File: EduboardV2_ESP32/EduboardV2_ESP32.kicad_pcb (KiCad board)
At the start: 2 copper layers, 30 x 51 mm, 19 parts, among them J1 Conn_02x26_Odd_Even, Q1 S8050_C139514, Q2 S8050_C139514, SW1 K2-1102SP-C4SC-04, SW2 K2-1102SP-C4SC-04, U1 ESP32-WROOM-E, U2 FT2232HL, U3 M93C46-WMN6TP

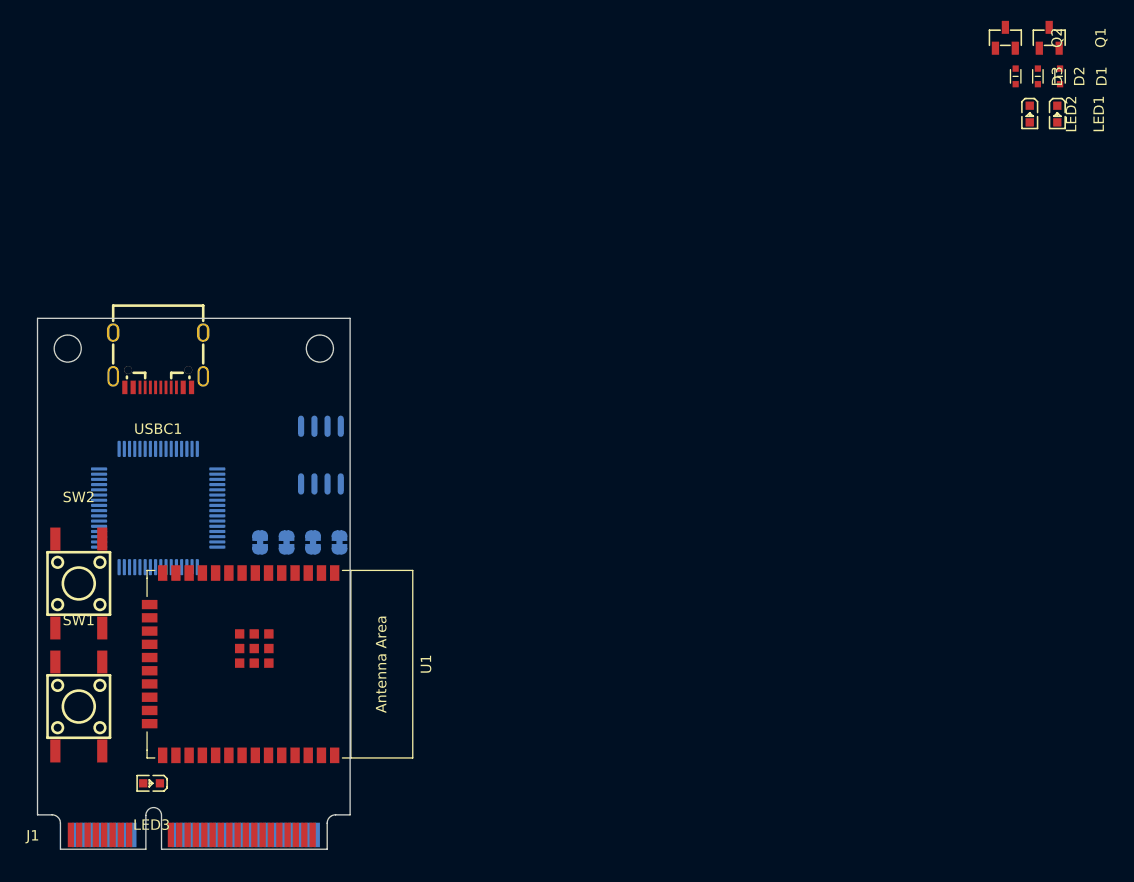
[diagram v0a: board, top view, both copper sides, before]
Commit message: all parts placed. descision about usb-debug line to be made...
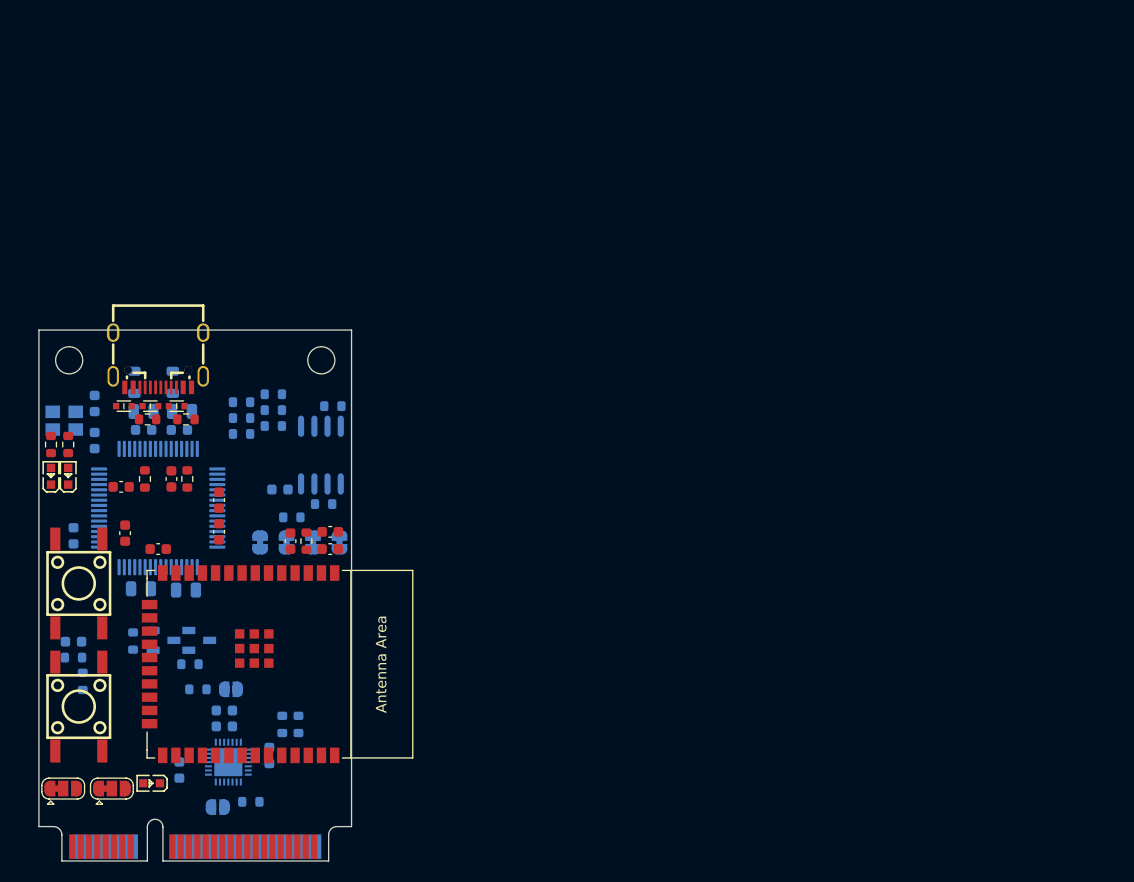
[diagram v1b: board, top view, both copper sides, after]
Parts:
- added C1: 12p, Capacitor_SMD:C_0603_1608Metric, B.Cu at (109.7, 113.5)
- added C10: 100n, Capacitor_SMD:C_0603_1608Metric, F.Cu at (117.1, 120.8)
- added C11: 100n, Capacitor_SMD:C_0603_1608Metric, F.Cu at (112.3, 121.5)
- added C12: 100n, Capacitor_SMD:C_0603_1608Metric, B.Cu at (107.7, 126.2)
- added C13: 100n, Capacitor_SMD:C_0603_1608Metric, F.Cu at (112.6, 126.0)
- added C14: 100n, Capacitor_SMD:C_0603_1608Metric, F.Cu at (121.7, 122.8)
- added C15: 100n, Capacitor_SMD:C_0603_1608Metric, F.Cu at (121.7, 125.9)
- added C16: 100n, Capacitor_SMD:C_0603_1608Metric, F.Cu at (115.8, 127.5)
- added C17: 100n, Capacitor_SMD:C_0603_1608Metric, F.Cu at (128.5, 126.7)
- added C18: 100n, Capacitor_SMD:C_0603_1608Metric, B.Cu at (107.7, 136.4)
- added C19: 100n, Capacitor_SMD:C_0603_1608Metric, F.Cu at (132.3, 127.5)
- added C2: 12p, Capacitor_SMD:C_0603_1608Metric, B.Cu at (109.7, 117.1)
- added C20: 1u, Capacitor_SMD:C_0603_1608Metric, F.Cu at (132.3, 125.9)
- added C21: 1u, Capacitor_SMD:C_0603_1608Metric, B.Cu at (122.2, 143.0)
- added C22: 100n, Capacitor_SMD:C_0603_1608Metric, B.Cu at (122.2, 144.5)
- added C23: 100n, Capacitor_SMD:C_0603_1608Metric, B.Cu at (117.9, 148.7)
- added C24: 100n, Capacitor_SMD:C_0603_1608Metric, B.Cu at (126.5, 147.3)
- added C3: 100n, Capacitor_SMD:C_0603_1608Metric, B.Cu at (127.5, 121.8)
- added C4: 4u7, Capacitor_SMD:C_0805_2012Metric, B.Cu at (118.5, 131.4)
- added C5: 4u7, Capacitor_SMD:C_0805_2012Metric, B.Cu at (114.2, 131.3)
- added C6: 4u7, Capacitor_SMD:C_0805_2012Metric, B.Cu at (114.4, 114.3)
- added C7: 4u7, Capacitor_SMD:C_0805_2012Metric, B.Cu at (118.1, 114.3)
- added C8: 100n, Capacitor_SMD:C_0603_1608Metric, B.Cu at (117.9, 116.1)
- added C9: 100n, Capacitor_SMD:C_0603_1608Metric, B.Cu at (114.4, 116.1)
- added FB1: FerriteBead_Small, Inductor_SMD:L_0805_2012Metric, B.Cu at (117.2, 111.5)
- added FB2: FerriteBead_Small, Inductor_SMD:L_0805_2012Metric, B.Cu at (113.5, 111.5)
- added JP5: SolderJumper_2_Open, Jumper:SolderJumper-2_P1.3mm_Open_RoundedPad1.0x1.5mm, B.Cu at (121.5, 152.3)
- added JP6: SolderJumper_2_Open, Jumper:SolderJumper-2_P1.3mm_Open_RoundedPad1.0x1.5mm, B.Cu at (122.8, 141.0)
- added JP7: SolderJumper_3_Bridged12, Jumper:SolderJumper-3_P1.3mm_Bridged12_RoundedPad1.0x1.5mm, F.Cu at (111.4, 150.5)
- added JP8: SolderJumper_3_Bridged12, Jumper:SolderJumper-3_P1.3mm_Bridged12_RoundedPad1.0x1.5mm, F.Cu at (106.7, 150.5)
- added R1: 2k2, Resistor_SMD:R_0603_1608Metric, B.Cu at (132.6, 113.8)
- added R10: 33R, Resistor_SMD:R_0603_1608Metric, B.Cu at (123.8, 116.5)
- added R11: 33R, Resistor_SMD:R_0603_1608Metric, B.Cu at (123.8, 114.9)
- added R12: 33R, Resistor_SMD:R_0603_1608Metric, B.Cu at (123.8, 113.4)
- added R13: 2k2, Resistor_SMD:R_0603_1608Metric, F.Cu at (107.2, 117.5)
- added R14: 2k2, Resistor_SMD:R_0603_1608Metric, F.Cu at (105.5, 117.5)
- added R15: 0R, Resistor_SMD:R_0603_1608Metric, B.Cu at (129.3, 144.3)
- added R16: 0R, Resistor_SMD:R_0603_1608Metric, B.Cu at (127.7, 144.3)
- added R17: 10k, Resistor_SMD:R_0603_1608Metric, B.Cu at (113.4, 136.3)
- added R18: 10k, Resistor_SMD:R_0603_1608Metric, B.Cu at (118.9, 138.6)
- added R19: 10k, Resistor_SMD:R_0603_1608Metric, F.Cu at (130.0, 126.7)
- added R2: 10k, Resistor_SMD:R_0603_1608Metric, B.Cu at (126.9, 114.2)
- added R20: 10k, Resistor_SMD:R_0603_1608Metric, B.Cu at (107.7, 137.9)
- added R21: 0R, Resistor_SMD:R_0603_1608Metric, B.Cu at (131.7, 123.2)
- added R22: 2k2, Resistor_SMD:R_0603_1608Metric, B.Cu at (108.6, 140.2)
- added R23: 10k, Resistor_SMD:R_0603_1608Metric, B.Cu at (124.7, 151.8)
- added R24: 10k, Resistor_SMD:R_0603_1608Metric, B.Cu at (119.6, 141.0)
- added R3: 10k, Resistor_SMD:R_0603_1608Metric, B.Cu at (126.9, 112.6)
- added R4: 10k, Resistor_SMD:R_0603_1608Metric, B.Cu at (126.9, 115.7)
- added R5: 0R, Resistor_SMD:R_0603_1608Metric, B.Cu at (128.7, 124.5)
- added R6: 10k, Resistor_SMD:R_0603_1608Metric, F.Cu at (114.8, 115.1)
- added R7: 10k, Resistor_SMD:R_0603_1608Metric, F.Cu at (118.5, 115.1)
- added R8: 1k, Resistor_SMD:R_0603_1608Metric, F.Cu at (118.6, 120.8)
- added R9: 12k, Resistor_SMD:R_0603_1608Metric, F.Cu at (114.6, 120.8)
- added U4: SX1509BIULTRT, EduboardV2_kicadlib:QFN-28_L4.0-W4.0-P0.40-BL-EP, B.Cu at (122.6, 148.0)
- added Y2: 12MHz, Crystal:Crystal_SMD_3225-4Pin_3.2x2.5mm, B.Cu at (106.8, 115.2)
- J1: value Conn_02x26_Odd_Even -> EduboardV2 PCIE UP Board Connector; footprint mpcie:mini-PCIe_F1_Full -> EduboardV2_kicadlib:mini-PCIe_F1_Full
- Q1, Q2: moved to B.Cu
- moved LED1 101.1 mm to (107.2, 120.5), turned to 90 degrees
- moved LED2 100.2 mm to (105.5, 120.5), turned to 90 degrees
- moved Q1 100.0 mm to (119.8, 136.3), turned to 180 degrees
- moved Q2 99.4 mm to (116.3, 136.3), turned to 180 degrees
- moved D1 95.3 mm to (112.5, 113.8), turned to 0 degrees
- moved D3 88.9 mm to (115.1, 113.8), turned to 0 degrees
- moved D2 88.5 mm to (117.6, 113.8), turned to 180 degrees
- moved J1 1.14 mm to (115.5, 157.4)
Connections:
- J1 pad 1: unconnected-(J1-Pin_1-Pad1) -> GND
- J1 pad 10: unconnected-(J1-Pin_10-Pad10) -> USB_Debug_D-
- J1 pad 11: unconnected-(J1-Pin_11-Pad11) -> Net-(J1-UART0_UP_RX)
- J1 pad 12: unconnected-(J1-Pin_12-Pad12) -> USB_Debug_D+
- J1 pad 13: unconnected-(J1-Pin_13-Pad13) -> Net-(J1-UART1_RS485_TX)
- J1 pad 14: unconnected-(J1-Pin_14-Pad14) -> GND
- J1 pad 15: unconnected-(J1-Pin_15-Pad15) -> Net-(J1-UART1_RS485_RX)
- J1 pad 16: unconnected-(J1-Pin_16-Pad16) -> GPIO_RS485_DE
- J1 pad 17: unconnected-(J1-Pin_17-Pad17) -> ESP_TMS
- J1 pad 18: unconnected-(J1-Pin_18-Pad18) -> ESP_IO4
- J1 pad 19: unconnected-(J1-Pin_19-Pad19) -> ESP_TDI
- J1 pad 2: unconnected-(J1-Pin_2-Pad2) -> VBUS
- J1 pad 20: unconnected-(J1-Pin_20-Pad20) -> ESP_IO5
- J1 pad 21: unconnected-(J1-Pin_21-Pad21) -> ESP_TCK
- J1 pad 22: unconnected-(J1-Pin_22-Pad22) -> ESP_IO2
- J1 pad 23: unconnected-(J1-Pin_23-Pad23) -> ESP_TDO
- J1 pad 24: unconnected-(J1-Pin_24-Pad24) -> ESP_IO18
- J1 pad 25: unconnected-(J1-Pin_25-Pad25) -> GPIO_RotEnc_SW
- J1 pad 26: unconnected-(J1-Pin_26-Pad26) -> ESP_IO19
- J1 pad 27: unconnected-(J1-Pin_27-Pad27) -> ESP_IO33
- J1 pad 28: unconnected-(J1-Pin_28-Pad28) -> ESP_IO23
- J1 pad 29: unconnected-(J1-Pin_29-Pad29) -> ESP_IO27
- J1 pad 3: unconnected-(J1-Pin_3-Pad3) -> +5V
- J1 pad 30: unconnected-(J1-Pin_30-Pad30) -> ESP_IO22
- J1 pad 31: unconnected-(J1-Pin_31-Pad31) -> GPIO_PWM_R
- J1 pad 32: unconnected-(J1-Pin_32-Pad32) -> ESP_IO21
- J1 pad 33: unconnected-(J1-Pin_33-Pad33) -> GPIO_PWM_G
- J1 pad 34: unconnected-(J1-Pin_34-Pad34) -> ESP_IO0
- J1 pad 35: unconnected-(J1-Pin_35-Pad35) -> GPIO_PWM_B
- J1 pad 36: unconnected-(J1-Pin_36-Pad36) -> ESP_IO32
- J1 pad 37: unconnected-(J1-Pin_37-Pad37) -> GPIO_LED0
- J1 pad 38: unconnected-(J1-Pin_38-Pad38) -> ESP_IO25
- J1 pad 39: unconnected-(J1-Pin_39-Pad39) -> GPIO_LED1
- J1 pad 4: unconnected-(J1-Pin_4-Pad4) -> +5V
- J1 pad 40: unconnected-(J1-Pin_40-Pad40) -> ESP_IO35
- J1 pad 41: unconnected-(J1-Pin_41-Pad41) -> GPIO_LED2
- J1 pad 42: unconnected-(J1-Pin_42-Pad42) -> ESP_IO26
- J1 pad 43: unconnected-(J1-Pin_43-Pad43) -> GPIO_LED3
- J1 pad 44: unconnected-(J1-Pin_44-Pad44) -> ESP_IO36
- J1 pad 45: unconnected-(J1-Pin_45-Pad45) -> GPIO_LED4
- J1 pad 46: unconnected-(J1-Pin_46-Pad46) -> ESP_IO34
- J1 pad 47: unconnected-(J1-Pin_47-Pad47) -> GPIO_LED5
- J1 pad 48: unconnected-(J1-Pin_48-Pad48) -> ESP_IO39
- J1 pad 49: unconnected-(J1-Pin_49-Pad49) -> GPIO_LED6
- J1 pad 5: unconnected-(J1-Pin_5-Pad5) -> +3V3
- J1 pad 50: unconnected-(J1-Pin_50-Pad50) -> GPIO_SW2
- J1 pad 51: unconnected-(J1-Pin_51-Pad51) -> GPIO_LED7
- J1 pad 52: unconnected-(J1-Pin_52-Pad52) -> GPIO_SW3
- J1 pad 6: unconnected-(J1-Pin_6-Pad6) -> +3V3
- J1 pad 7: unconnected-(J1-Pin_7-Pad7) -> GND
- J1 pad 8: unconnected-(J1-Pin_8-Pad8) -> GND
- J1 pad 9: unconnected-(J1-Pin_9-Pad9) -> Net-(J1-UART0_UP_TX)
- U1 pad 10: unconnected-(U1-DAC_1/ADC2_CH8/GPIO25-Pad10) -> ESP_IO25
- U1 pad 11: unconnected-(U1-DAC_2/ADC2_CH9/GPIO26-Pad11) -> ESP_IO26
- U1 pad 12: unconnected-(U1-ADC2_CH7/GPIO27-Pad12) -> ESP_IO27
- U1 pad 24: unconnected-(U1-ADC2_CH2/GPIO2-Pad24) -> ESP_IO2
- U1 pad 26: unconnected-(U1-ADC2_CH0/GPIO4-Pad26) -> ESP_IO4
- U1 pad 27: unconnected-(U1-GPIO16-Pad27) -> ESP_IO16
- U1 pad 28: unconnected-(U1-GPIO17-Pad28) -> ESP_IO17
- U1 pad 29: unconnected-(U1-GPIO5-Pad29) -> ESP_IO5
- U1 pad 30: unconnected-(U1-GPIO18-Pad30) -> ESP_IO18
- U1 pad 31: unconnected-(U1-GPIO19-Pad31) -> ESP_IO19
- U1 pad 33: unconnected-(U1-GPIO21-Pad33) -> ESP_IO21
- U1 pad 36: unconnected-(U1-GPIO22-Pad36) -> ESP_IO22
- U1 pad 37: unconnected-(U1-GPIO23-Pad37) -> ESP_IO23
- U1 pad 4: unconnected-(U1-SENSOR_VP/GPIO36/ADC1_CH0-Pad4) -> ESP_IO36
- U1 pad 5: unconnected-(U1-SENSOR_VN/GPIO39/ADC1_CH3-Pad5) -> ESP_IO39
- U1 pad 6: unconnected-(U1-GPIO34/ADC1_CH6-Pad6) -> ESP_IO34
- U1 pad 7: unconnected-(U1-GPIO35/ADC1_CH7-Pad7) -> ESP_IO35
- U1 pad 8: unconnected-(U1-32K_XP/GPIO32/ADC1_CH4-Pad8) -> ESP_IO32
- U1 pad 9: unconnected-(U1-32K_XN/GPIO33/ADC1_CH5-Pad9) -> ESP_IO33
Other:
- board size 30 x 51 mm -> 30 x 50.9 mm
